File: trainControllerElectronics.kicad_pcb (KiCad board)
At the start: 2 copper layers, 109.8 x 94.4 mm, 35 parts, among them J1 0541324062, J2 USB4135-GF-A, J3 B2B-PH-K-S, J4 Pin header 2.54 1x03, J5 Pin socket 2.54 1x03, Q1 BSS670S2LH6327XTSA1, SW1 PTS647SM38SMTR2 LFS, SW10 PTS647SM38SMTR2 LFS, SW11 PTS647SM38SMTR2 LFS, SW12 PTS647SM38SMTR2 LFS, SW2 PTS647SM38SMTR2 LFS, SW3 PTS647SM38SMTR2 LFS, SW4 PTS647SM38SMTR2 LFS, SW5 PTS647SM38SMTR2 LFS, SW6 PTS647SM38SMTR2 LFS, SW7 PTS647SM38SMTR2 LFS, SW8 PTS647SM38SMTR2 LFS, SW9 PTS647SM38SMTR2 LFS, U1 CD74HC4067M96, U2 ZXM64P03XTA, U3 MCP73831T-2ACI/OT

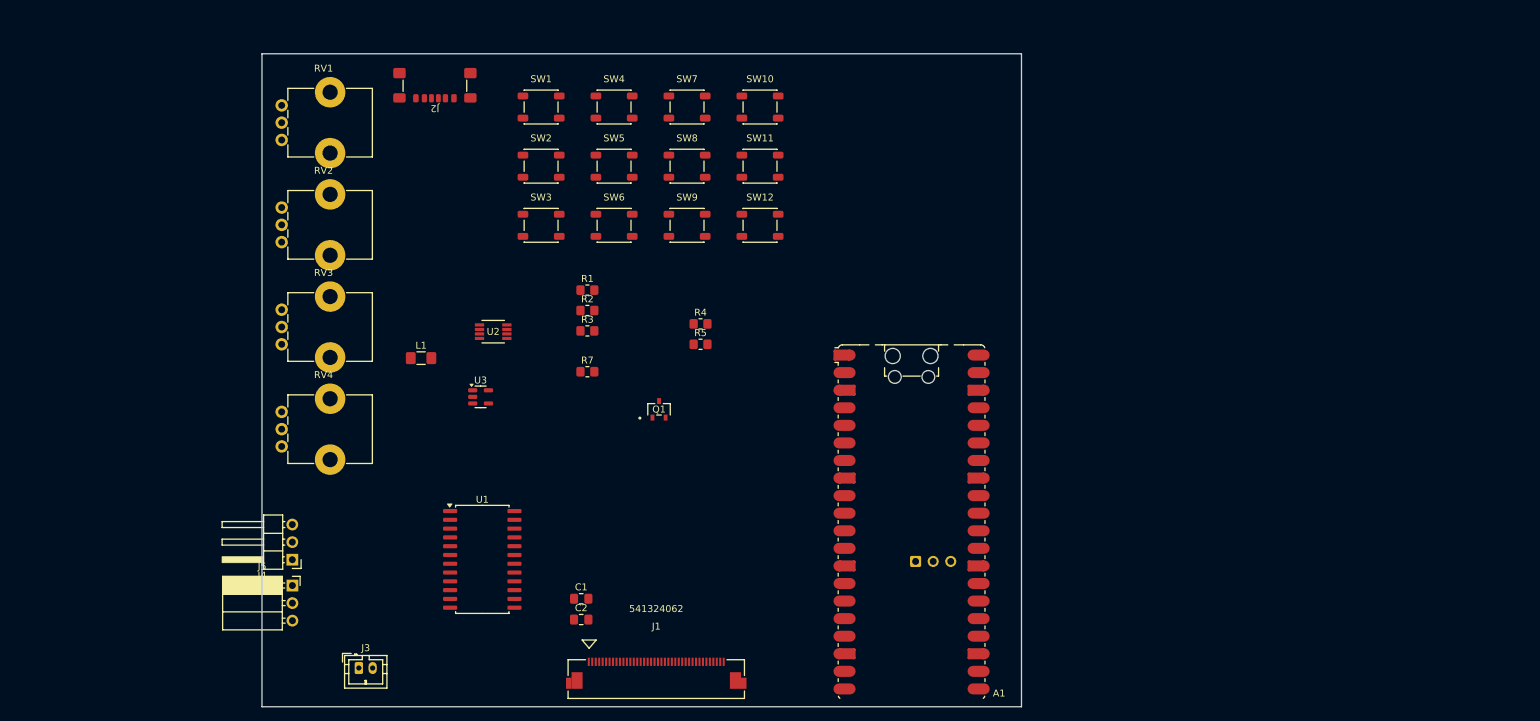
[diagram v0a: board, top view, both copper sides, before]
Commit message: PCB ready
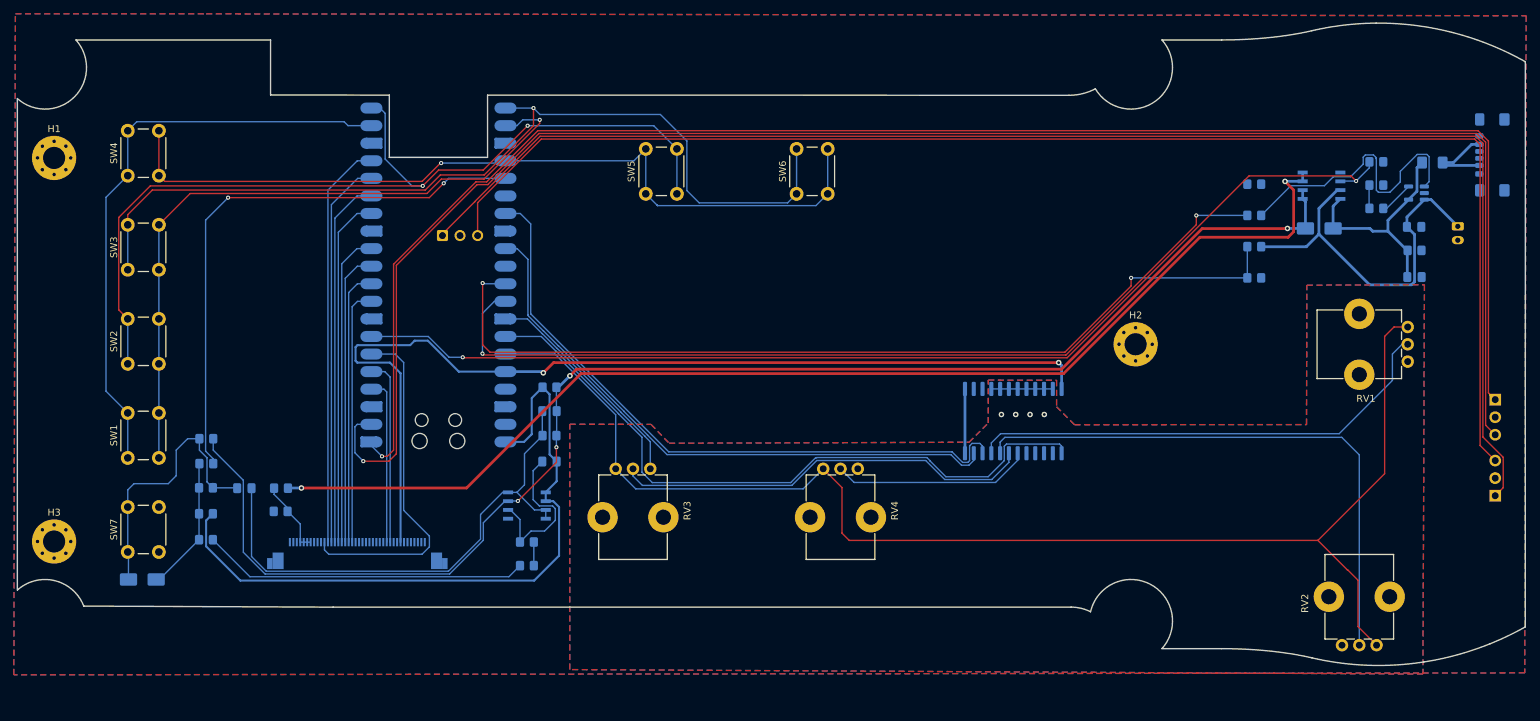
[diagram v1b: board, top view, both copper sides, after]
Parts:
- removed A1: SC0918 RaspberryPi Pico W, Module:RaspberryPi_Pico_W_SMD_HandSolder
- removed Q1: BSS670S2LH6327XTSA1, BSS670S2L:PG-SOT23-3-5_INF
- removed SW10, SW11, SW12, SW8, SW9: PTS647SM38SMTR2 LFS, Button_Switch_SMD:SW_SPST_PTS647_Sx38
- added C3: 10u, Capacitor_SMD:C_0805_2012Metric_Pad1.18x1.45mm_HandSolder, B.Cu at (115.6, 101.5)
- added C4: 0.1u, Capacitor_SMD:C_0805_2012Metric_Pad1.18x1.45mm_HandSolder, B.Cu at (115.6, 94.3)
- added C5: 1u, Capacitor_SMD:C_0805_2012Metric_Pad1.18x1.45mm_HandSolder, B.Cu at (71.5, 105.4)
- added D1: SS15, Diode_SMD:D_SMA, B.Cu at (226.8, 67.8)
- added D2: SS15, Diode_SMD:D_SMA, B.Cu at (56.7, 118.6)
- added H1: MountingHole, MountingHole:MountingHole_3.2mm_M3_Pad_Via, F.Cu at (43.9, 57.7)
- added H2: MountingHole, MountingHole:MountingHole_3.2mm_M3_Pad_Via, F.Cu at (200.3, 84.6)
- added H3: MountingHole, MountingHole:MountingHole_3.2mm_M3_Pad_Via, F.Cu at (43.9, 113.1)
- added R10: 1K, Resistor_SMD:R_0805_2012Metric_Pad1.20x1.40mm_HandSolder, B.Cu at (235.1, 61.6)
- added R11: 0R, Resistor_SMD:R_0805_2012Metric_Pad1.20x1.40mm_HandSolder, B.Cu at (115.6, 90.8)
- added R12: 100K, Resistor_SMD:R_0805_2012Metric_Pad1.20x1.40mm_HandSolder, B.Cu at (65.9, 109.1)
- added R13: 100K, Resistor_SMD:R_0805_2012Metric_Pad1.20x1.40mm_HandSolder, B.Cu at (115.6, 97.8)
- added R14: 10K, Resistor_SMD:R_0805_2012Metric_Pad1.20x1.40mm_HandSolder, B.Cu at (66.0, 98.2)
- added R15: 1K, Resistor_SMD:R_0805_2012Metric_Pad1.20x1.40mm_HandSolder, B.Cu at (66.0, 101.8)
- added R16: 100K, Resistor_SMD:R_0805_2012Metric_Pad1.20x1.40mm_HandSolder, B.Cu at (65.9, 112.8)
- added R17: 100K, Resistor_SMD:R_0805_2012Metric_Pad1.20x1.40mm_HandSolder, B.Cu at (112.3, 116.6)
- added R18: 100K, Resistor_SMD:R_0805_2012Metric_Pad1.20x1.40mm_HandSolder, B.Cu at (112.3, 113.2)
- added R19: 0R, Resistor_SMD:R_0805_2012Metric_Pad1.20x1.40mm_HandSolder, B.Cu at (65.9, 105.3)
- added R6: 0R, Resistor_SMD:R_0805_2012Metric_Pad1.20x1.40mm_HandSolder, B.Cu at (76.7, 108.8)
- added R8: 10K, Resistor_SMD:R_0805_2012Metric_Pad1.20x1.40mm_HandSolder, B.Cu at (240.6, 71.0)
- added R9: 10K, Resistor_SMD:R_0805_2012Metric_Pad1.20x1.40mm_HandSolder, B.Cu at (235.1, 58.2)
- added REF**: OSHW-Logo2_9.8x8mm_SilkScreen, Symbol:OSHW-Logo2_9.8x8mm_SilkScreen, B.Cu at (160.2, 83.2)
- added U4: IRF7319TRPBF, IRF7319:TRANS_IRF7103TRPBF_INF, B.Cu at (227.2, 61.7)
- added U5: IRF7319TRPBF, IRF7319:TRANS_IRF7103TRPBF_INF, B.Cu at (112.3, 107.9)
- C1, C2, L1, R1, R3, R4, U1, U3: moved to B.Cu
- J1: value 0541324062 -> Pin socket 2.54 1x03; footprint WM3436CT-ND‎:CON_541324062_MOL -> Connector_PinSocket_2.54mm:PinSocket_1x03_P2.54mm_Horizontal; moved to B.Cu
- J2: value USB4135-GF-A -> Pin header 2.54 1x03; footprint Connector_USB:USB_C_Receptacle_GCT_USB4135-GF-A_6P_TopMnt_Horizontal -> Connector_PinHeader_2.54mm:PinHeader_1x03_P2.54mm_Horizontal; moved to B.Cu
- J3: value B2B-PH-K-S -> 0541324062; footprint Connector_JST:JST_PH_B2B-PH-K_1x02_P2.00mm_Vertical -> WM3436CT-ND‎:CON_541324062_MOL; moved to B.Cu
- J4: value Pin header 2.54 1x03 -> USB4135-GF-A; footprint Connector_PinHeader_2.54mm:PinHeader_1x03_P2.54mm_Horizontal -> Connector_USB:USB_C_Receptacle_GCT_USB4135-GF-A_6P_TopMnt_Horizontal; moved to B.Cu
- J5: value Pin socket 2.54 1x03 -> B2B-PH-K-S; footprint Connector_PinSocket_2.54mm:PinSocket_1x03_P2.54mm_Horizontal -> Connector_JST:JST_PH_B2B-PH-K_1x02_P2.00mm_Vertical; moved to B.Cu
- R2: value 2K -> 10K; moved to B.Cu
- R5: value 10K -> 0R; moved to B.Cu
- R7: value 0R -> 1K; moved to B.Cu
- SW1, SW2, SW3, SW4, SW5, SW6, SW7: value PTS647SM38SMTR2 LFS -> 1825910-6; footprint Button_Switch_SMD:SW_SPST_PTS647_Sx38 -> Button_Switch_THT:SW_PUSH_6mm
- U2: value ZXM64P03XTA -> SC0918 RaspberryPi Pico W; footprint ZXM64P03XTA:SOIC8_ZXM64P03X_DIO -> Module:RaspberryPi_Pico_W_SMD_HandSolder; moved to B.Cu
- moved J4 184.2 mm to (253.0, 57.2), turned to -90 degrees
- moved J5 176.3 mm to (246.9, 67.5), turned to -90 degrees
- moved RV2 168.7 mm to (235.1, 128.1), turned to 90 degrees
- moved RV1 165.0 mm to (239.6, 82.1), turned to 180 degrees
- moved J2 164.8 mm to (252.3, 106.5), turned to 0 degrees
- moved L1 148.9 mm to (243.2, 58.3), turned to 180 degrees
- moved U3 138.5 mm to (240.9, 62.7), turned to 180 degrees
- moved C2 133.1 mm to (240.6, 67.6)
- moved C1 129.1 mm to (240.6, 74.9)
- moved J1 127.8 mm to (252.3, 92.6), turned to 180 degrees
- moved R7 116.5 mm to (235.1, 65.0)
- moved SW7 103.3 mm to (54.6, 114.6), turned to 90 degrees
- moved R2 97.4 mm to (217.4, 66.0)
- moved R3 96.7 mm to (217.4, 75.0), turned to 180 degrees
- moved R1 96.6 mm to (217.4, 70.5)
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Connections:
- C1 pad 1: Vbus -> Net-(D1-A)
- C2 pad 1: BATT -> Vbat
- J1 pad 1: GND -> UART0_TX
- J1 pad 2: unconnected-(J1-Pad2) -> GND
- J1 pad 3: unconnected-(J1-Pad3) -> UART0_RX
- J3 pad 1: BATT -> GND
- J3 pad 2: GND -> unconnected-(J3-Pad2)
- J5 pad 1: UART0_TX -> Vbat
- L1 pad 1: Net-(J2-VBUS-PadA9) -> Net-(J4-VBUS-PadA9)
- L1 pad 2: Vbus -> Net-(D1-A)
- R1 pad 1: GND -> Net-(U2-GPIO26_ADC0)
- R1 pad 2: Vbus -> Vbat
- R2 pad 1: GND -> Net-(U2-GPIO27_ADC1)
- R2 pad 2: Net-(U3-PROG) -> BATT_STAT
- R3 pad 1: Backlight_PWM -> GND
- R3 pad 2: GND -> Net-(U2-GPIO26_ADC0)
- R4 pad 1: Net-(A1-GPIO27_ADC1) -> GND
- R4 pad 2: BATT -> Net-(U2-GPIO27_ADC1)
- R5 pad 1: GND -> Net-(J3-Pad34)
- R5 pad 2: Net-(A1-GPIO27_ADC1) -> Backlight_Cathode
- R7 pad 1: Net-(Q1-D) -> Net-(R10-Pad2)
- R7 pad 2: GND -> Net-(U3-PROG)
- SW2 pad 1: KEY_COL_1 -> KEY_COL_2
- SW2 pad 2: KEY_ROW_2 -> KEY_ROW_1
- SW3 pad 1: KEY_COL_1 -> KEY_COL_3
- SW3 pad 2: KEY_ROW_3 -> KEY_ROW_1
- SW4 pad 2: KEY_ROW_4 -> KEY_ROW_2
- SW5 pad 2: KEY_ROW_1 -> KEY_ROW_2
- SW6 pad 1: KEY_COL_2 -> KEY_COL_3
- SW7 pad 1: KEY_COL_2 -> Net-(D2-K)
- SW7 pad 2: KEY_ROW_3 -> GND
- U1 pad 1: ADC0 -> ADC2
- U1 pad 16: GND -> AGND
- U1 pad 17: GND -> AGND
- U1 pad 18: GND -> AGND
- U1 pad 19: GND -> AGND
- U1 pad 2: GND -> AGND
- U1 pad 20: GND -> AGND
- U1 pad 21: GND -> AGND
- U1 pad 22: GND -> AGND
- U1 pad 23: GND -> AGND
- U1 pad 3: GND -> AGND
- U1 pad 4: GND -> AGND
- U1 pad 5: GND -> AGND
- U2 pad 1: BATT -> UART0_TX
- U2 pad 2: BATT -> UART0_RX
- U2 pad 3: BATT -> GND
- U2 pad 4: Vbus -> Display_WR
- U2 pad 5: Vsys -> Display_DC
- U2 pad 6: Vsys -> Display_RST
- U2 pad 7: Vsys -> Backlight_PWM
- U2 pad 8: Vsys -> GND
- U3 pad 3: BATT -> Vbat
- U3 pad 4: Vbus -> Net-(D1-A)
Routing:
- net UART0_RX: track 0.00 -> 249.2 mm, vias 0 -> 1
- net UART0_TX: track 0.00 -> 236.3 mm, vias 0 -> 1
- net SWCK: track 0.00 -> 209.5 mm
- net Net-(D1-K): track 0.00 -> 207.4 mm, vias 0 -> 4
- net SWIO: track 0.00 -> 200.4 mm
- net ADC_VREF: track 0.00 -> 195.5 mm
- net Backlight_Cathode: track 0.00 -> 172.4 mm, vias 0 -> 2
- net Backlight_PWM: track 0.00 -> 160.7 mm, vias 0 -> 2
- net +3.3V: track 0.00 -> 142.2 mm, vias 0 -> 2
- net KEY_COL_3: track 0.00 -> 133.5 mm, vias 0 -> 1
- net Net-(U2-GPIO26_ADC0): track 0.00 -> 132.9 mm, vias 0 -> 2
- net KEY_COL_2: track 0.00 -> 131.7 mm, vias 0 -> 2
- net Net-(U2-GPIO27_ADC1): track 0.00 -> 129.7 mm, vias 0 -> 2
- net KEY_ROW_2: track 0.00 -> 121.6 mm, vias 0 -> 1
- net KEY_ROW_1: track 0.00 -> 100.6 mm, vias 0 -> 1
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- added copper zone on B.Cu, net AGND
- added copper zone on F.Cu, net AGND
- added copper zone on B.Cu, net GND
- added copper zone on F.Cu, net GND
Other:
- board size 109.8 x 94.4 mm -> 218 x 92.9 mm
- board text added: "Black -"
- board text added: "CAUTION Inverting battery polarity may cause fire or explossion"
- board text added: "RED +"
- board text added: "Rick's Train controller Version 1.0"
